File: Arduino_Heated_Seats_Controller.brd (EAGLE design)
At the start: 41.6 x 35.7 mm, 22 parts, among them U1 ATMEGA328P-AU, U2 UA78M05CDCY, U3 ULN2003ADE4, U4 IC_TD62783-SO-18W

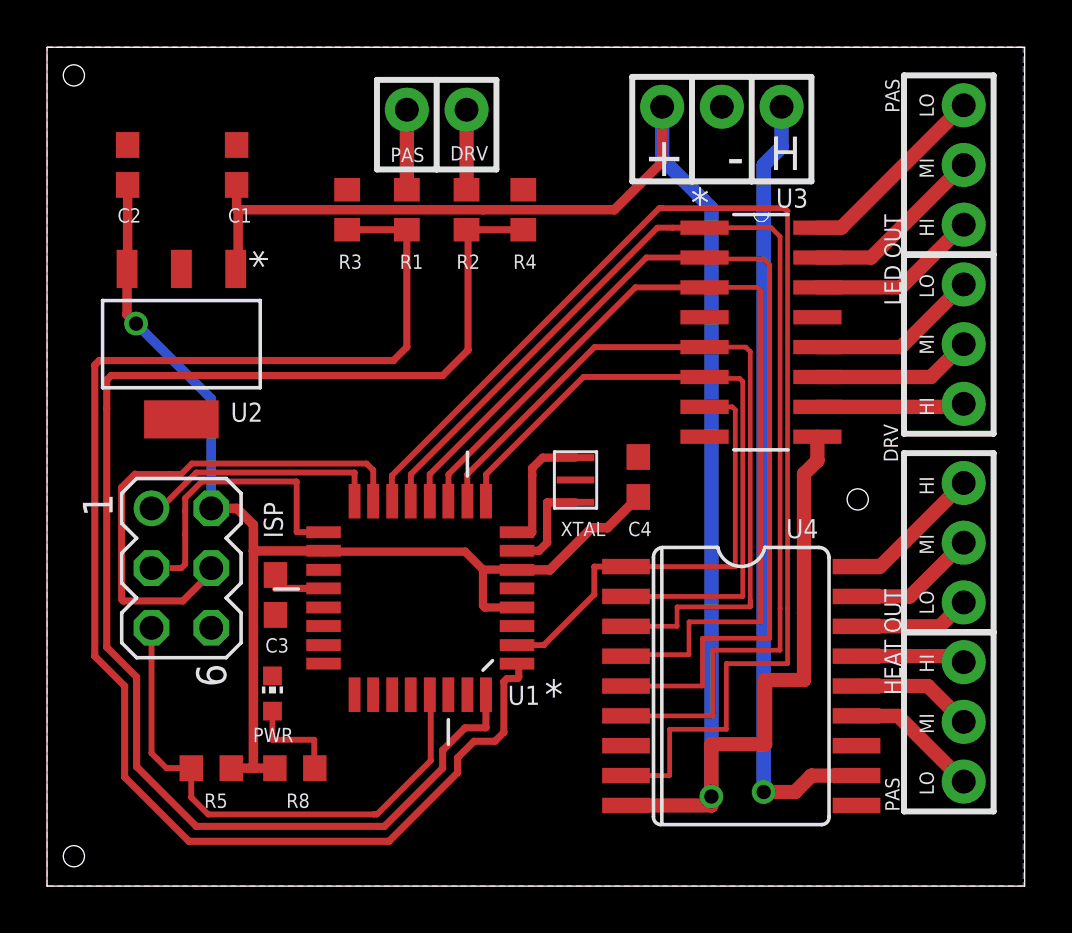
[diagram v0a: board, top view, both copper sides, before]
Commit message: Changes from freelancer.com - lovely~
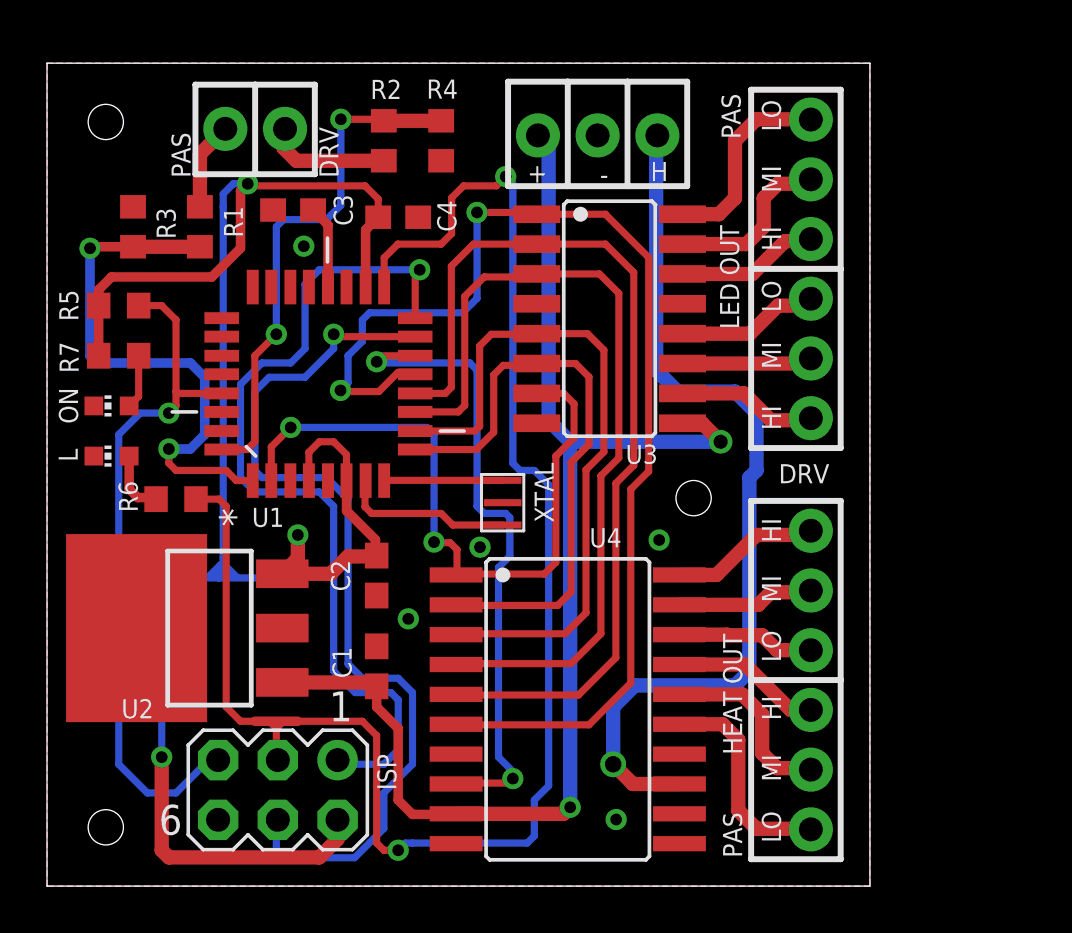
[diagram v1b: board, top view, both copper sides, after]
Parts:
- removed PWR: (no value), led:CHIP-LED0603
- removed R8: 1k, resistor:R0603
- added L, ON: (no value), led:CHIP-LED0603
- added R6, R7: 1K, resistor:R0603
- R1, R2: value 15k -> 15K
- R3, R4, R5: value 10k -> 10K
- U2: value UA78M05CDCY -> UA78M05; device Texas Instruments_By_element14_Batch_1:SOT230P700X180-4N -> Roylib Regulator:SOT223
- U3: value ULN2003ADE4 -> TPL7407L; device Texas Instruments_By_element14_Batch_1:SOIC127P600X175-16N -> Roylib Drivers:SOIC16N
- U4: value IC_TD62783-SO-18W -> A2982; device dp_devices:SO-18L -> Roylib Drivers:SOIC20W
- moved C1 22.1 mm to (14.0, 9.35)
- moved C2 20.4 mm to (14.0, 13.2), turned to 270 degrees
- moved R5 20.1 mm to (3.05, 24.7), turned to 0 degrees
- moved C3 16.4 mm to (10.5, 28.8), turned to 180 degrees
- moved C4 15.0 mm to (14.9, 28.4), turned to 0 degrees
- moved U2 12.1 mm to (6.91, 11.0), turned to 90 degrees
- moved ISP 10.3 mm to (9.82, 4.09), turned to 180 degrees
- moved U3 10.2 mm to (23.9, 24.1)
- moved U1 10.1 mm to (11.5, 21.4), turned to 90 degrees
- moved U$1 10.0 mm to (20.1, 15.3)
- moved R3 9.13 mm to (3.66, 28.0)
- moved R1 8.83 mm to (6.50, 28.0)
- moved BTN-IN 7.76 mm to (7.58, 32.2)
- moved U4 7.56 mm to (22.1, 7.52), turned to 0 degrees
- moved H-OUT 6.81 mm to (32.5, 15.1)
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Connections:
- new net N$1: L.A, R6.2
- net D13: now also R6.1
- net DH-HIGH: now also U4.20; no longer U4.18
- net DH-LOW: now also U4.18; no longer U4.16
- net DH-MID: now also U4.19; no longer U4.17
- net GND: now also L.C, ON.C, U4.12; no longer PWR.C, U2.4, U4.10
- net H-ON: now also U4.13; no longer U4.11
- net N$3: now also ON.A, R7.2; no longer PWR.A, R8.2
- net PH-HIGH: now also U4.17; no longer U4.15
- net PH-LOW: now also U4.15; no longer U4.13
- net PH-MID: now also U4.16; no longer U4.14
- net VDD: now also R7.1; no longer R8.1
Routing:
- net D13: track 12.6 -> 70.1 mm, vias 0 -> 2
- net D3: track 62.2 -> 23.2 mm, vias 0 -> 2
- net D2: track 59.9 -> 22.1 mm, vias 0 -> 2
- net VDD: track 50.6 -> 85.5 mm, vias 1 -> 3
- net D12: track 10.5 -> 37.1 mm, vias 0 -> 1
- net D10: track 53.6 -> 27.8 mm, vias 0 -> 2
- net VIN: track 79.1 -> 54.5 mm, vias 1 -> 2
- net D11: track 21.8 -> 39.1 mm, vias 0 -> 1
- net D4: track 19.4 -> 28.8 mm, vias 0 -> 2
- net RESET: track 22.8 -> 29.8 mm, vias 0 -> 1
- net H-ON: track 33.7 -> 38.2 mm
- net D8: track 43.6 -> 39.6 mm
- net PH-LOW: track 5.72 -> 9.20 mm
- net D7: track 39.0 -> 35.6 mm
- net D6: track 32.7 -> 29.4 mm
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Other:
- board size 41.6 x 35.7 mm -> 35 x 35 mm
- board text added: "Arduino Powered Heated Seat Controller Rev. 4b"
- board text added: "https://goo.gl/t2CsID"
- board text removed: "Arduino Powered Heated Seat Controller rev. 4a"
- board text removed: "https://github.com/avluis/ArduinoHeatedSeatController-Hardware"
